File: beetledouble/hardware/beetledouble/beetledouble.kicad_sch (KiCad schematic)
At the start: 29 parts, among them J1 XT30PW-M, J2 rxin, J6 prog connector, U1 78L12G-AB3-R, U2 DD4012SB, U3 ATtiny1614-SS

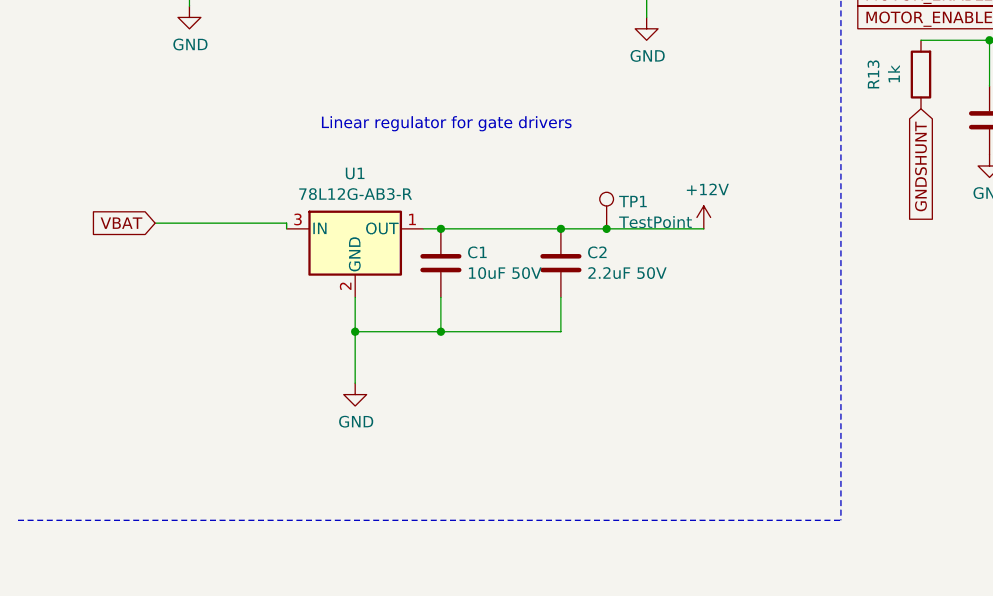
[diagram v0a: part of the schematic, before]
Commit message: update pcb
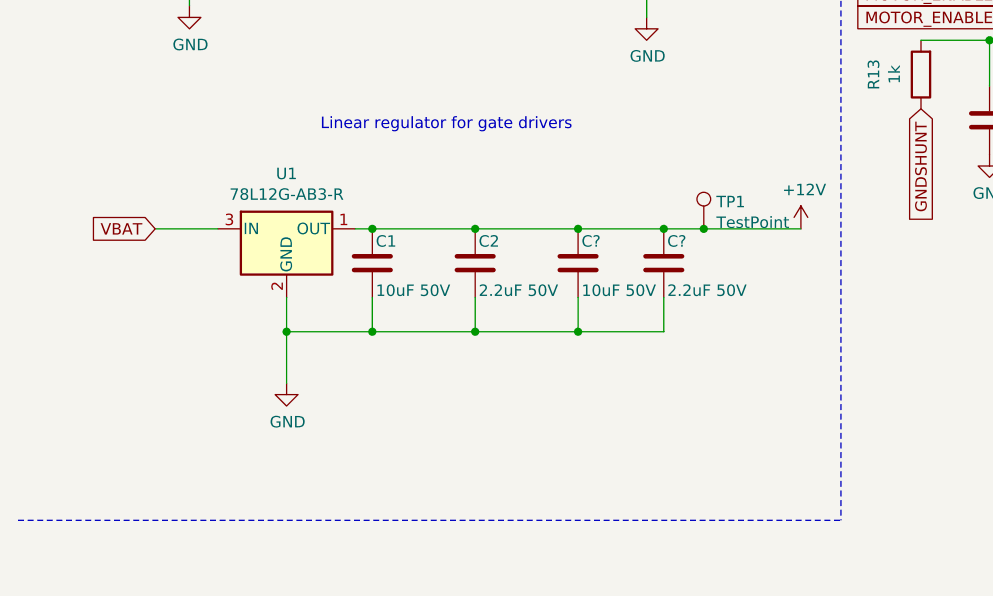
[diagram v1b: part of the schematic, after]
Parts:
- added C?: 2.2uF 50V, Capacitor_SMD:C_0603_1608Metric, symbol Device:C
- added C?: 10uF 50V, Capacitor_SMD:C_1206_3216Metric, symbol Device:C
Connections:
- net +12V: now also C?.1, C?.1
- net GND: now also C?.2, C?.2
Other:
- moved on the sheet: C1, C2, TP1, U1
